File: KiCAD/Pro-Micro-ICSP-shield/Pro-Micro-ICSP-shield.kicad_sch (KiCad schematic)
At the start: 13 parts, among them J1 Pro Micro, J2 ICSP, SW1 MODE, SW2 RESET

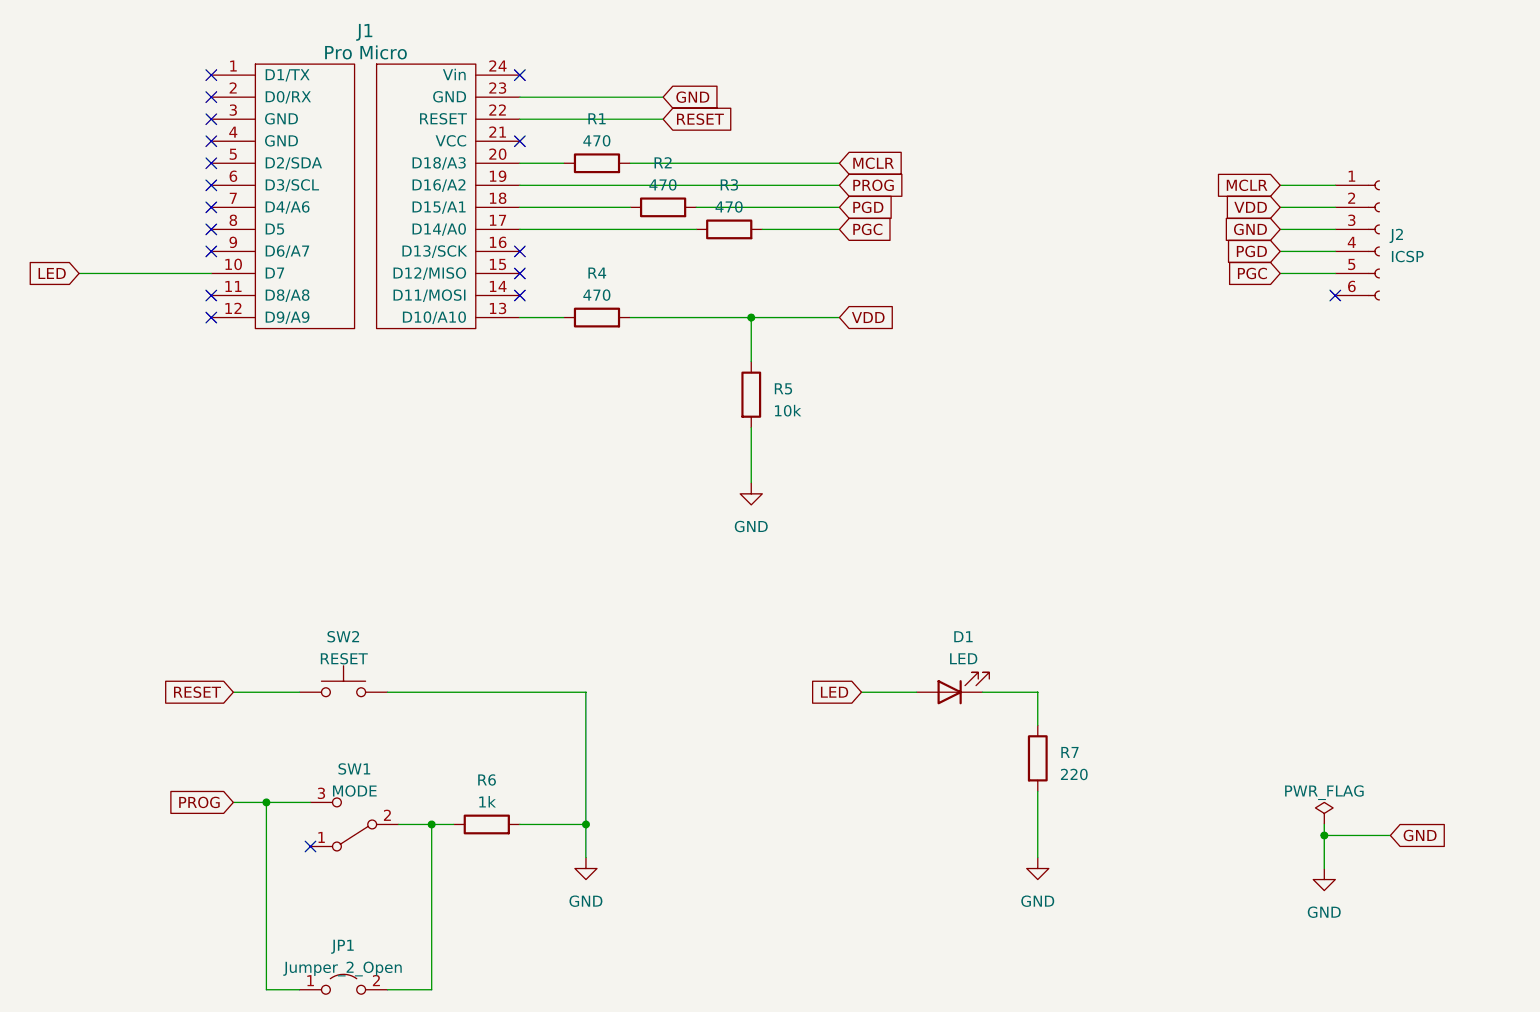
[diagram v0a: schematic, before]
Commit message: Add Pro-Micro-ICSP-shield-1.1
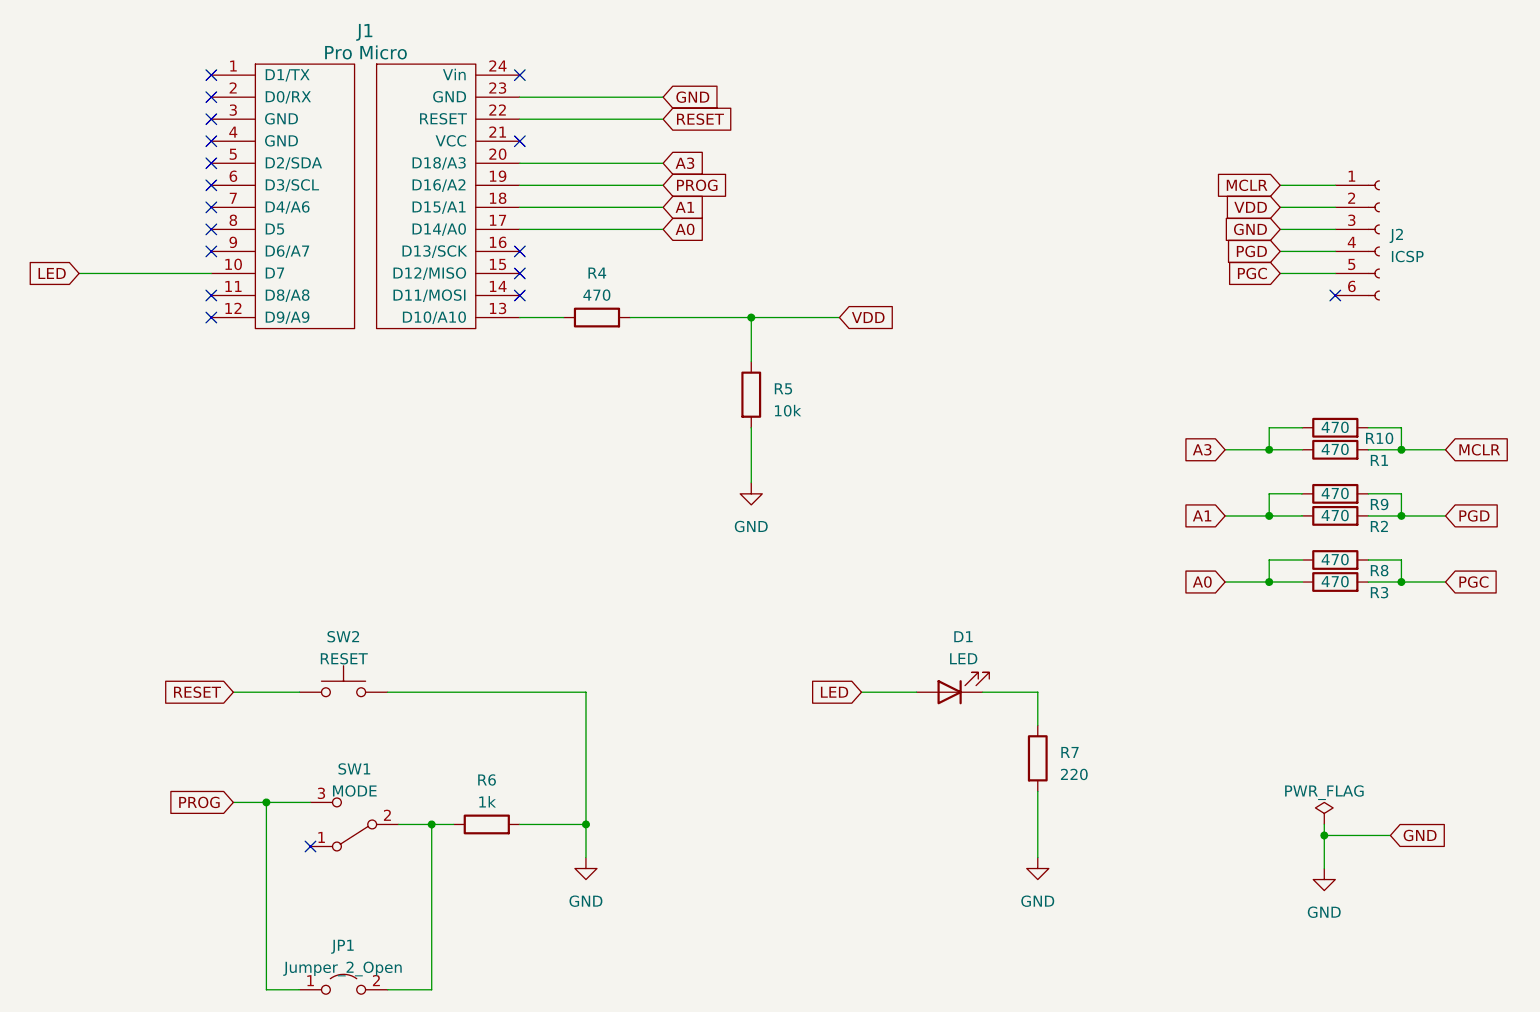
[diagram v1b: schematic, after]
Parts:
- added R10, R8, R9: 470, Resistor_THT:R_Axial_DIN0207_L6.3mm_D2.5mm_P10.16mm_Horizontal, symbol Device:R
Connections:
- net MCLR: now also R10.2
- net PGC: now also R8.2
- net PGD: now also R9.2
- net A1: now reaches J1.18 (D15/A1), R2.1
- net A1: now also R9.1
- net A0: now reaches J1.17 (D14/A0), R3.1
- net A0: now also R8.1
- net A3: now reaches J1.20 (D18/A3), R1.1
- net A3: now also R10.1
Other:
- moved on the sheet: R1, R2, R3
